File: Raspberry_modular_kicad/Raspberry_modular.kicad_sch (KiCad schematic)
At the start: 21 parts, among them J1 Raspberry_Pi_2_3, U1 MCP3008, U3 MCP3008

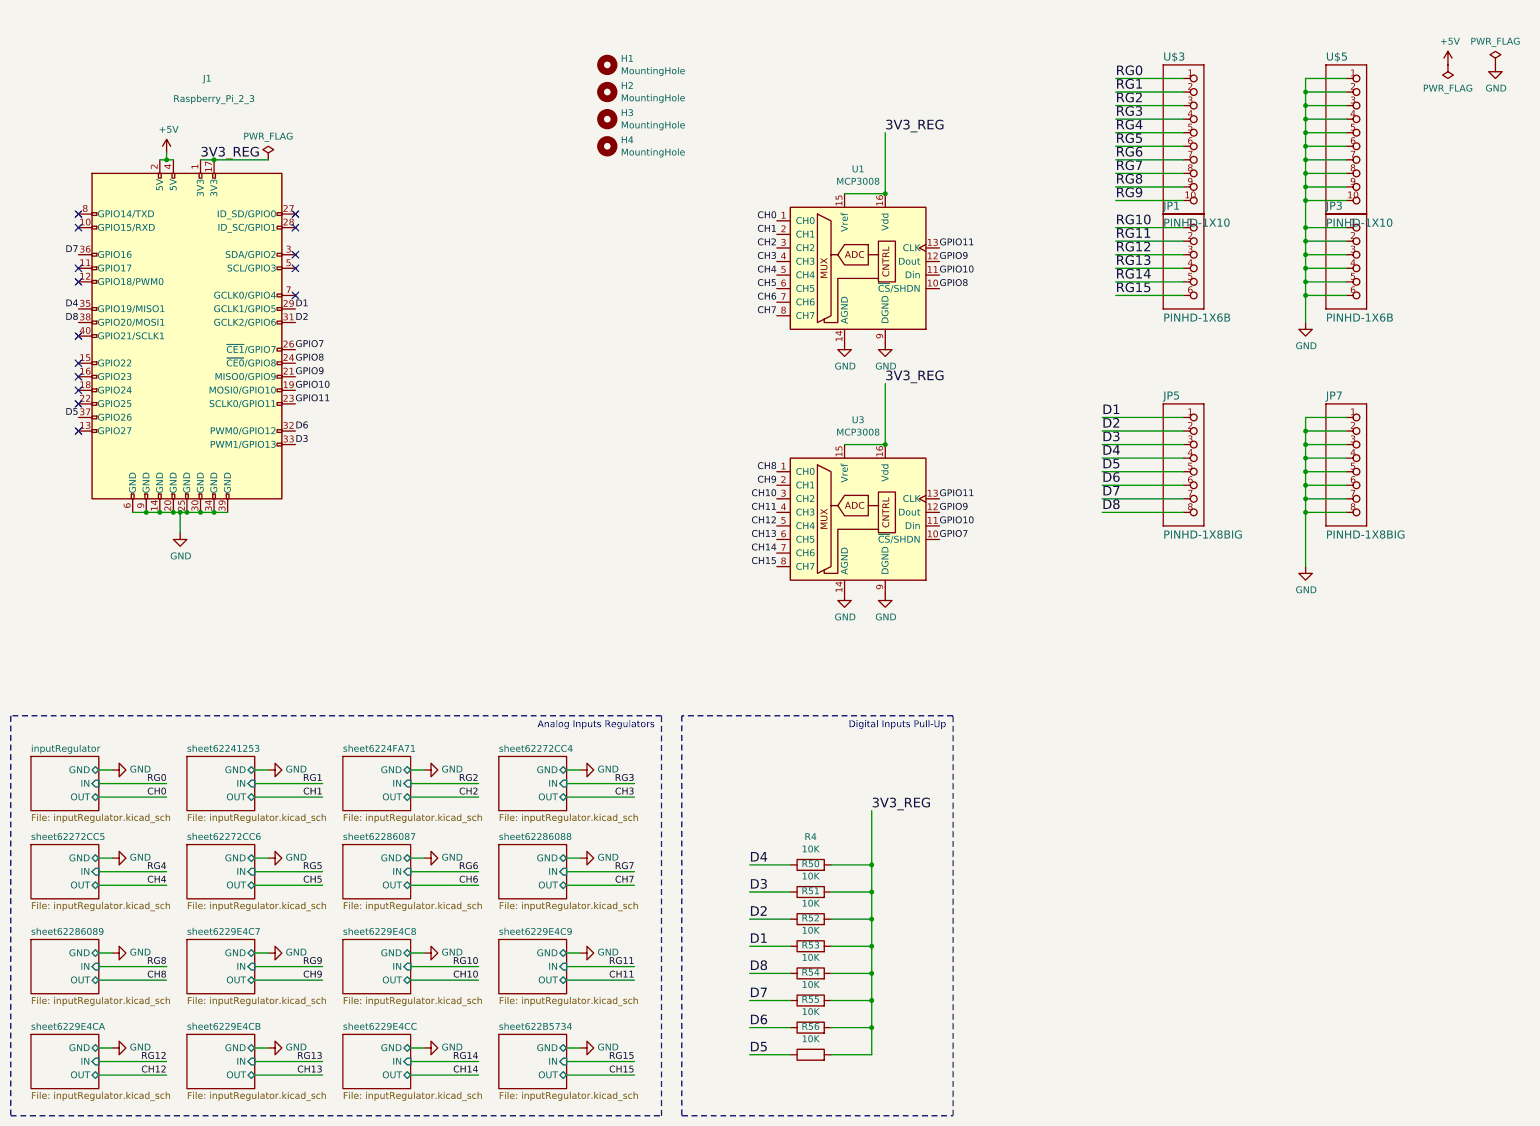
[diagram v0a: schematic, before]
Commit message: [UDPT] Shematics
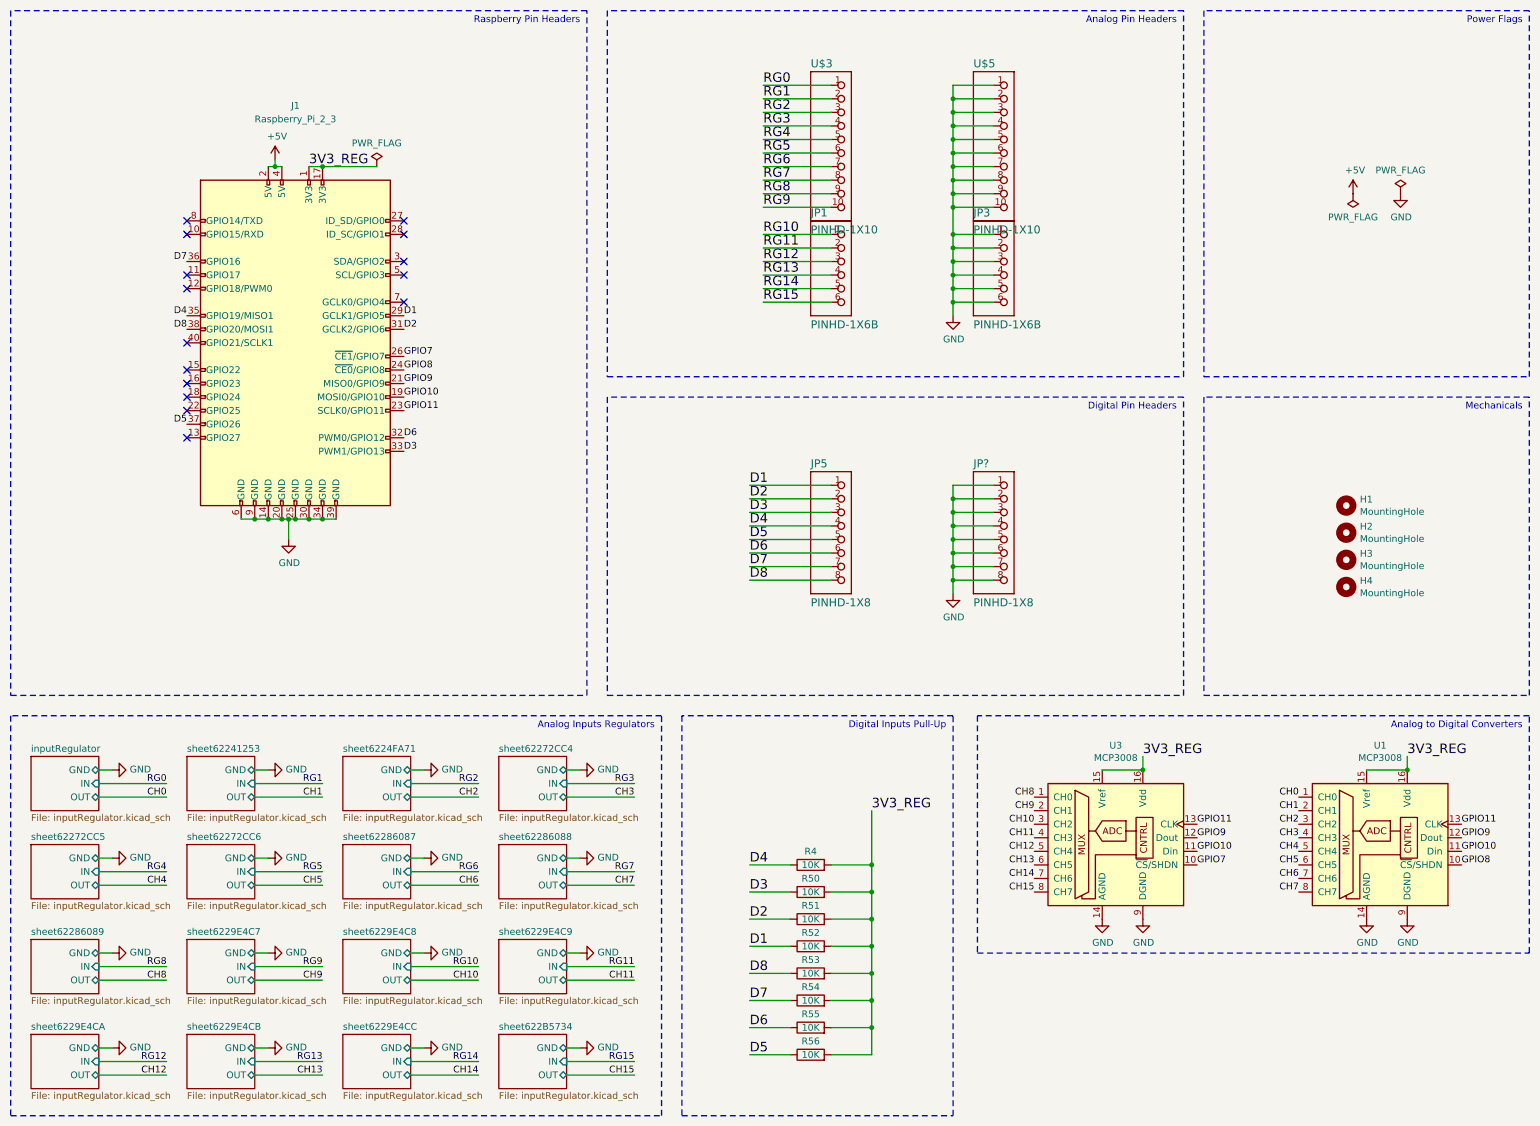
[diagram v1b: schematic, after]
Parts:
- JP5: value PINHD-1X8BIG -> PINHD-1X8; symbol Raspberry_modular-rescue:PINHD-1X8BIG-OhEye-eagle-import -> Modular Shield:PINHD-1X8
- JP?: renamed from JP7; value PINHD-1X8BIG -> PINHD-1X8; symbol Raspberry_modular-rescue:PINHD-1X8BIG-OhEye-eagle-import -> Modular Shield:PINHD-1X8
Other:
- note added: "Analog Pin Headers"
- note added: "Analog to Digital Converters"
- note added: "Digital Pin Headers"
- note added: "Mechanicals"
- note added: "Power Flags"
- note added: "Raspberry Pin Headers"
- moved on the sheet: H1, H2, H3, H4, J1, JP1, JP3, JP5, JP?, U$3, U$5, U1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
